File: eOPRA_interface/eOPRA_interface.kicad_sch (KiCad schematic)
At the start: 20 parts, among them J1 CONN_01X04_MALE, J2 CONN_01X04_MALE, J3 CONN_01X04_MALE, J4 CONN_01X02_MALE, J5 CONN_01X04_MALE, J6 CONN_02X10, J8 CONN_01X04_MALE, Q5 Q_PMOS_GSD, U1 ARM-SWD-10, U10 USB_C_2.0, U27 Mounting-holes, U28 Mounting-holes, U5 XT-X, U7 Mounting-holes, U8 Mounting-holes

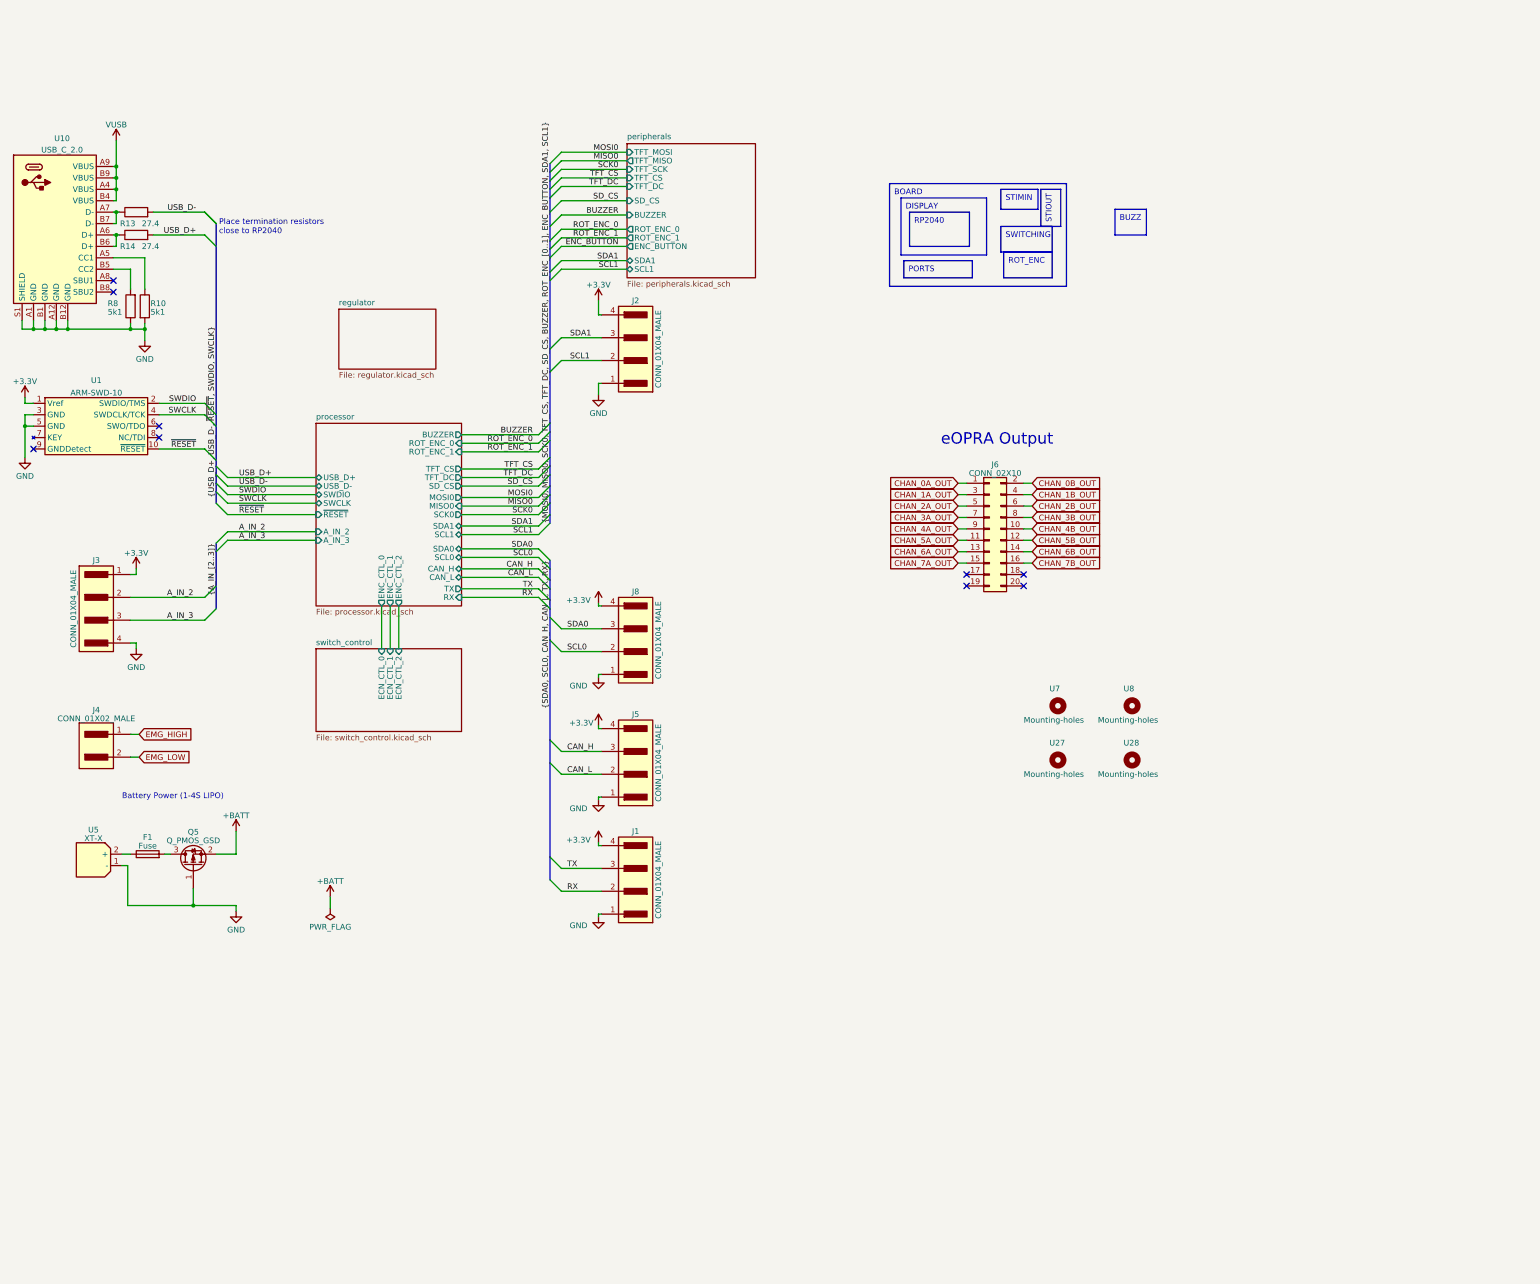
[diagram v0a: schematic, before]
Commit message: draft 2 wifi finish
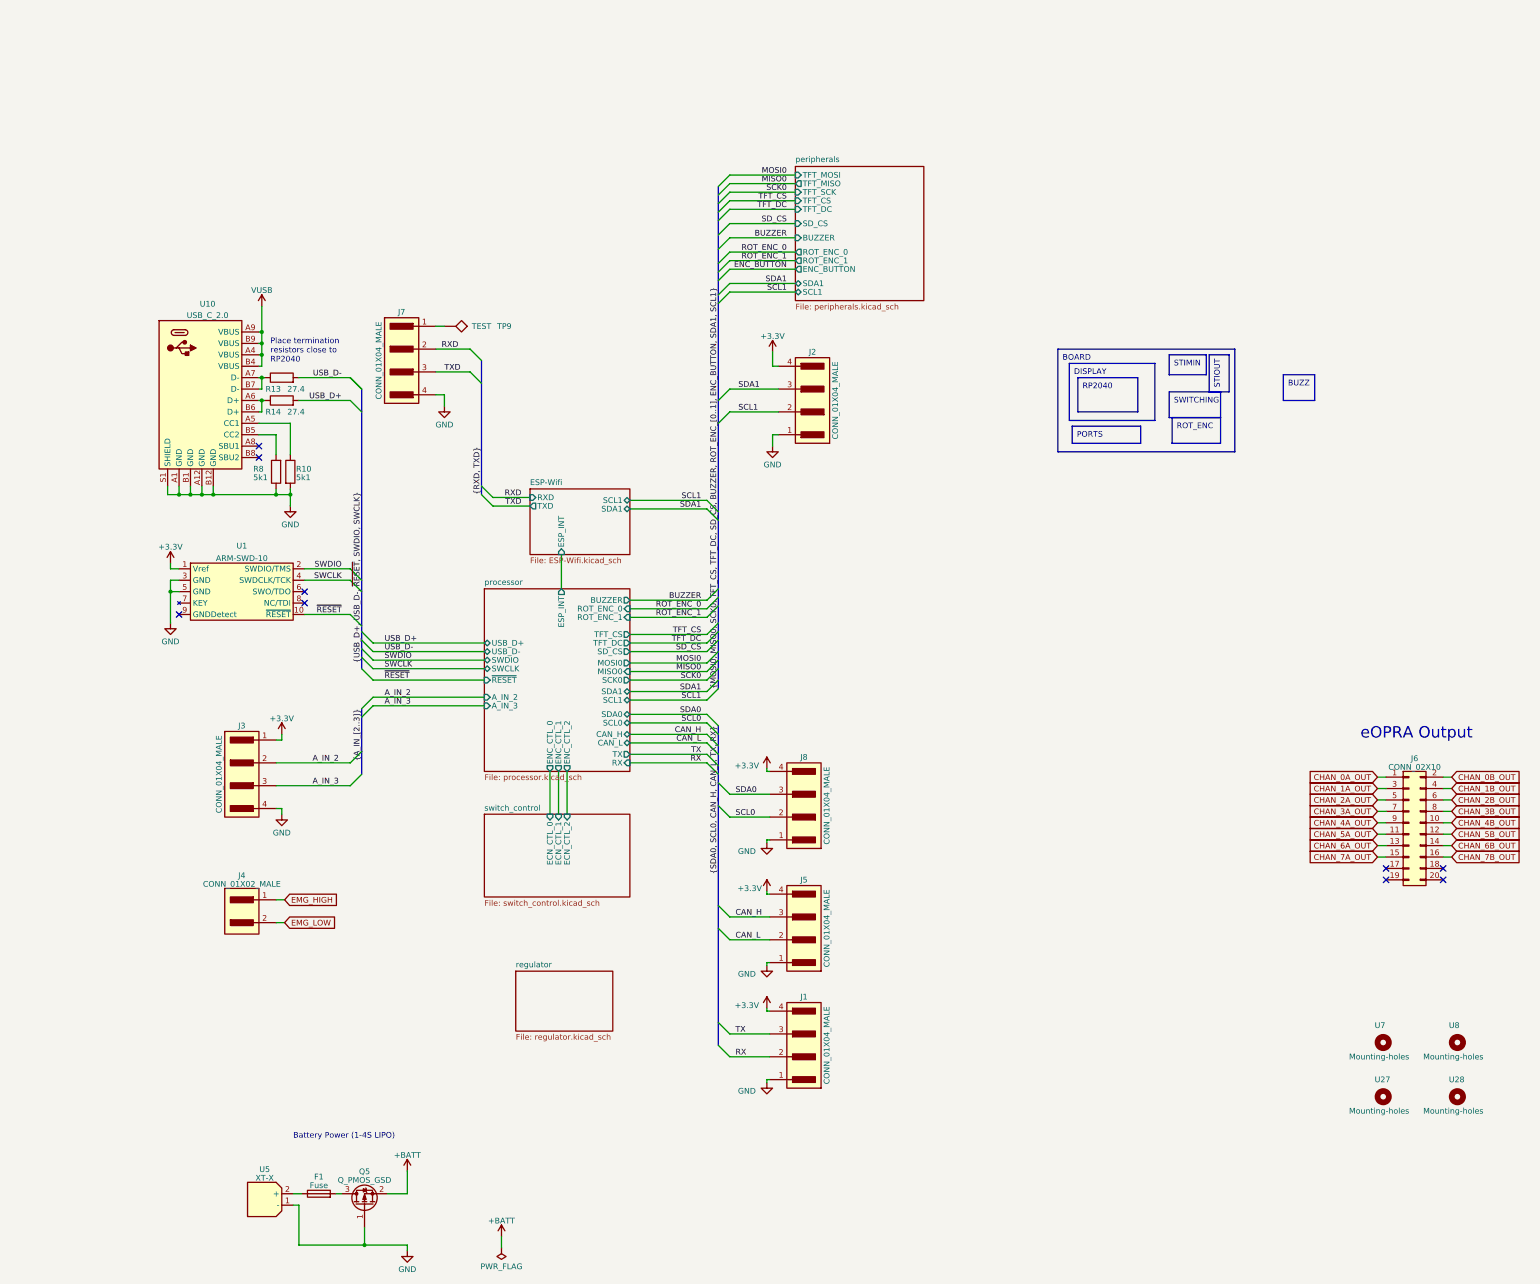
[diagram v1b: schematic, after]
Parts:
- added J7: CONN_01X04_MALE, project_footprints:JST_SM04B-GHS-TB(LF)(SN)-, symbol 5.connector.interconnect:CONN_01X04_MALE
- added TP9: TEST, 0_misc:test_point_1.0mm_square, symbol 5.connector.interconnect:TEST
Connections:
- net GND: now also J7.4
- new net: J7.1, TP9.1
- new net RXD: J7.2
- new net TXD: J7.3
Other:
- added sheet ESP-Wifi (ESP-Wifi.kicad_sch)
- sheet processor ports: added ESP_INT; removed none
- moved on the sheet: F1, J1, J2, J3, J4, J5, J6, J8, Q5, R10, R13, R14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
